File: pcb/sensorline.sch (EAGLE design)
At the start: 31 parts, among them X1 52745-1290

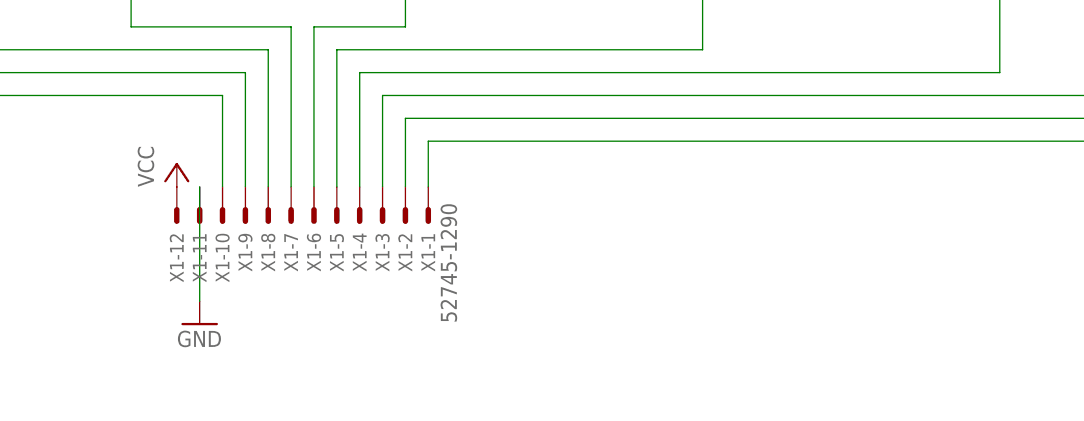
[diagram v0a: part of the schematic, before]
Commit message: a takie tam poprawki
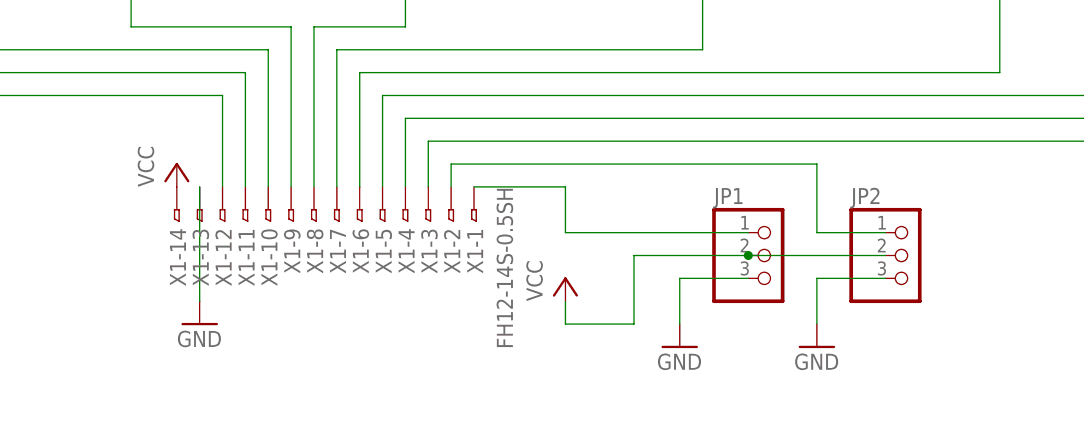
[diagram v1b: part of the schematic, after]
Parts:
- added JP1, JP2: (no value), pinhead:PINHD-1X3
- X1: value 52745-1290 -> FH12-14S-0.5SH; device con-molex:52745-1290 -> con-hirose:FH12-14S-0.5SH
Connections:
- new net N$21: JP1.1, X1-1.1
- new net N$22: JP2.1, X1-2.1
- net GND: now also JP1.3, JP2.3, X1-13.1; no longer X1-11.S
- net N$10: now also X1-8.1; no longer X1-6.S
- net N$12: now also X1-7.1; no longer X1-5.S
- net N$14: now also X1-6.1; no longer X1-4.S
- net N$16: now also X1-5.1; no longer X1-3.S
- net N$18: now also X1-4.1; no longer X1-2.S
- net N$2: now also X1-12.1; no longer X1-10.S
- net N$20: now also X1-3.1; no longer X1-1.S
- net N$4: now also X1-11.1; no longer X1-9.S
- net N$6: now also X1-10.1; no longer X1-8.S
- net N$8: now also X1-9.1; no longer X1-7.S
- net VCC: now also JP1.2, JP2.2, X1-14.1; no longer X1-12.S
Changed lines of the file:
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@@
 <?xml version="1.0" encoding="utf-8"?>
 <!DOCTYPE eagle SYSTEM "eagle.dtd">
-<eagle version="7.1.0">
+<eagle version="8.1.1">
 <drawing>
 <settings>
@@
 <part name="GND10" library="supply1" deviceset="GND" device=""/>
 <part name="P+10" library="supply1" deviceset="VCC" device=""/>
-<part name="X1" library="con-molex" deviceset="52745-1290" device=""/>
 <part name="P+11" library="supply1" deviceset="VCC" device=""/>
 <part name="GND11" library="supply1" deviceset="GND" device=""/>
 <part name="FRAME1" library="frames" deviceset="DINA3_L" device=""/>
+<part name="X1" library="con-hirose" deviceset="FH12-14S-0.5S" device="H"/>
+<part name="JP1" library="pinhead" deviceset="PINHD-1X3" device=""/>
+<part name="JP2" library="pinhead" deviceset="PINHD-1X3" device=""/>
+<part name="P+12" library="supply1" deviceset="VCC" device=""/>
+<part name="GND12" library="supply1" deviceset="GND" device=""/>
+<part name="GND13" library="supply1" deviceset="GND" device=""/>
 </parts>
 <sheets>
@@
 <instance part="GND10" gate="1" x="251.46" y="78.74"/>
 <instance part="P+10" gate="VCC" x="251.46" y="119.38"/>
-<instance part="X1" gate="-1" x="109.22" y="45.72" rot="R270"/>
-<instance part="X1" gate="-2" x="106.68" y="45.72" rot="R270"/>
-<instance part="X1" gate="-3" x="104.14" y="45.72" rot="R270"/>
-<instance part="X1" gate="-4" x="101.6" y="45.72" rot="R270"/>
-<instance part="X1" gate="-5" x="99.06" y="45.72" rot="R270"/>
-<instance part="X1" gate="-6" x="96.52" y="45.72" rot="R270"/>
-<instance part="X1" gate="-7" x="93.98" y="45.72" rot="R270"/>
-<instance part="X1" gate="-8" x="91.44" y="45.72" rot="R270"/>
-<instance part="X1" gate="-9" x="88.9" y="45.72" rot="R270"/>
-<instance part="X1" gate="-10" x="86.36" y="45.72" rot="R270"/>
-<instance part="X1" gate="-11" x="83.82" y="45.72" rot="R270"/>
-<instance part="X1" gate="-12" x="81.28" y="45.72" rot="R270"/>
 <instance part="P+11" gate="VCC" x="81.28" y="50.8"/>
 <instance part="GND11" gate="1" x="83.82" y="33.02"/>
 <instance part="FRAME1" gate="G$1" x="-78.74" y="-60.96"/>
 <instance part="FRAME1" gate="G$2" x="208.28" y="-60.96"/>
+<instance part="X1" gate="-1" x="114.3" y="45.72" rot="R270"/>
+<instance part="X1" gate="-2" x="111.76" y="45.72" rot="R270"/>
+<instance part="X1" gate="-3" x="109.22" y="45.72" rot="R270"/>
+<instance part="X1" gate="-4" x="106.68" y="45.72" rot="R270"/>
+<instance part="X1" gate="-5" x="104.14" y="45.72" rot="R270"/>
+<instance part="X1" gate="-6" x="101.6" y="45.72" rot="R270"/>
+<instance part="X1" gate="-7" x="99.06" y="45.72" rot="R270"/>
+<instance part="X1" gate="-8" x="96.52" y="45.72" rot="R270"/>
+<instance part="X1" gate="-9" x="93.98" y="45.72" rot="R270"/>
+<instance part="X1" gate="-10" x="91.44" y="45.72" rot="R270"/>
+<instance part="X1" gate="-11" x="88.9" y="45.72" rot="R270"/>
+<instance part="X1" gate="-12" x="86.36" y="45.72" rot="R270"/>
+<instance part="X1" gate="-13" x="83.82" y="45.72" rot="R270"/>
+<instance part="X1" gate="-14" x="81.28" y="45.72" rot="R270"/>
+<instance part="JP1" gate="A" x="147.32" y="40.64"/>
+<instance part="JP2" gate="A" x="162.56" y="40.64"/>
+<instance part="P+12" gate="VCC" x="124.46" y="38.1"/>
+<instance part="GND12" gate="1" x="137.16" y="30.48"/>
+<instance part="GND13" gate="1" x="152.4" y="30.48"/>
 </instances>
 <busses>
@@
 <junction x="-38.1" y="99.06"/>
 <wire x1="-25.4" y1="99.06" x2="-25.4" y2="58.42" width="0.1524" layer="91"/>
-<pinref part="X1" gate="-10" pin="S"/>
 <wire x1="-25.4" y1="58.42" x2="86.36" y2="58.42" width="0.1524" layer="91"/>
 <wire x1="86.36" y1="58.42" x2="86.36" y2="48.26" width="0.1524" layer="91"/>
+<pinref part="X1" gate="-12" pin="1"/>
 </segment>
 </net>
@@
 </segment>
 <segment>
-<pinref part="X1" gate="-11" pin="S"/>
 <pinref part="GND11" gate="1" pin="GND"/>
 <wire x1="83.82" y1="48.26" x2="83.82" y2="35.56" width="0.1524" layer="91"/>
+<pinref part="X1" gate="-13" pin="1"/>
+</segment>
+<segment>
+<pinref part="JP1" gate="A" pin="3"/>
+<wire x1="144.78" y1="38.1" x2="137.16" y2="38.1" width="0.1524" layer="91"/>
+<wire x1="137.16" y1="38.1" x2="137.16" y2="33.02" width="0.1524" layer="91"/>
+<pinref part="GND12" gate="1" pin="GND"/>
+</segment>
+<segment>
+<pinref part="JP2" gate="A" pin="3"/>
+<wire x1="160.02" y1="38.1" x2="152.4" y2="38.1" width="0.1524" layer="91"/>
+<wire x1="152.4" y1="38.1" x2="152.4" y2="33.02" width="0.1524" layer="91"/>
+<pinref part="GND13" gate="1" pin="GND"/>
 </segment>
 </net>
@@
 </segment>
 <segment>
-<pinref part="X1" gate="-12" pin="S"/>
 <pinref part="P+11" gate="VCC" pin="VCC"/>
+<pinref part="X1" gate="-14" pin="1"/>
+</segment>
+<segment>
+<pinref part="JP2" gate="A" pin="2"/>
+<pinref part="JP1" gate="A" pin="2"/>
+<wire x1="160.02" y1="40.64" x2="144.78" y2="40.64" width="0.1524" layer="91"/>
+<wire x1="144.78" y1="40.64" x2="132.08" y2="40.64" width="0.1524" layer="91"/>
+<wire x1="132.08" y1="40.64" x2="132.08" y2="33.02" width="0.1524" layer="91"/>
+<junction x="144.78" y="40.64"/>
+<wire x1="132.08" y1="33.02" x2="124.46" y2="33.02" width="0.1524" layer="91"/>
+<wire x1="124.46" y1="33.02" x2="124.46" y2="35.56" width="0.1524" layer="91"/>
+<pinref part="P+12" gate="VCC" pin="VCC"/>
 </segment>
 </net>
@@
 <junction x="-5.08" y="99.06"/>
 <wire x1="7.62" y1="99.06" x2="7.62" y2="60.96" width="0.1524" layer="91"/>
-<pinref part="X1" gate="-9" pin="S"/>
 <wire x1="7.62" y1="60.96" x2="88.9" y2="60.96" width="0.1524" layer="91"/>
 <wire x1="88.9" y1="60.96" x2="88.9" y2="48.26" width="0.1524" layer="91"/>
+<pinref part="X1" gate="-11" pin="1"/>
 </segment>
 </net>
@@
 <junction x="27.94" y="99.06"/>
 <wire x1="40.64" y1="99.06" x2="40.64" y2="63.5" width="0.1524" layer="91"/>
-<pinref part="X1" gate="-8" pin="S"/>
 <wire x1="40.64" y1="63.5" x2="91.44" y2="63.5" width="0.1524" layer="91"/>
 <wire x1="91.44" y1="63.5" x2="91.44" y2="48.26" width="0.1524" layer="91"/>
+<pinref part="X1" gate="-10" pin="1"/>
 </segment>
 </net>
@@
 <junction x="60.96" y="99.06"/>
 <wire x1="76.2" y1="99.06" x2="76.2" y2="66.04" width="0.1524" layer="91"/>
-<pinref part="X1" gate="-7" pin="S"/>
 <wire x1="76.2" y1="66.04" x2="93.98" y2="66.04" width="0.1524" layer="91"/>
 <wire x1="93.98" y1="66.04" x2="93.98" y2="48.26" width="0.1524" layer="91"/>
+<pinref part="X1" gate="-9" pin="1"/>
 </segment>
 </net>
@@
 <junction x="93.98" y="99.06"/>
 <wire x1="106.68" y1="99.06" x2="106.68" y2="66.04" width="0.1524" layer="91"/>
-<pinref part="X1" gate="-6" pin="S"/>
 <wire x1="106.68" y1="66.04" x2="96.52" y2="66.04" width="0.1524" layer="91"/>
 <wire x1="96.52" y1="66.04" x2="96.52" y2="48.26" width="0.1524" layer="91"/>
+<pinref part="X1" gate="-8" pin="1"/>
 </segment>
 </net>
@@
 <junction x="127" y="99.06"/>
 <wire x1="139.7" y1="99.06" x2="139.7" y2="63.5" width="0.1524" layer="91"/>
-<pinref part="X1" gate="-5" pin="S"/>
 <wire x1="139.7" y1="63.5" x2="99.06" y2="63.5" width="0.1524" layer="91"/>
 <wire x1="99.06" y1="63.5" x2="99.06" y2="48.26" width="0.1524" layer="91"/>
+<pinref part="X1" gate="-7" pin="1"/>
 </segment>
 </net>
@@
 <wire x1="172.72" y1="60.96" x2="101.6" y2="60.96" width="0.1524" layer="91"/>
 <wire x1="101.6" y1="60.96" x2="101.6" y2="48.26" width="0.1524" layer="91"/>
-<pinref part="X1" gate="-4" pin="S"/>
+<pinref part="X1" gate="-6" pin="1"/>
 </segment>
 </net>
@@
 <junction x="193.04" y="99.06"/>
 <wire x1="205.74" y1="99.06" x2="205.74" y2="58.42" width="0.1524" layer="91"/>
-<pinref part="X1" gate="-3" pin="S"/>
 <wire x1="205.74" y1="58.42" x2="104.14" y2="58.42" width="0.1524" layer="91"/>
 <wire x1="104.14" y1="58.42" x2="104.14" y2="48.26" width="0.1524" layer="91"/>
+<pinref part="X1" gate="-5" pin="1"/>
 </segment>
 </net>
@@
 <junction x="226.06" y="99.06"/>
 <wire x1="238.76" y1="99.06" x2="238.76" y2="55.88" width="0.1524" layer="91"/>
-<pinref part="X1" gate="-2" pin="S"/>
 <wire x1="238.76" y1="55.88" x2="106.68" y2="55.88" width="0.1524" layer="91"/>
 <wire x1="106.68" y1="55.88" x2="106.68" y2="48.26" width="0.1524" layer="91"/>
+<pinref part="X1" gate="-4" pin="1"/>
 </segment>
 </net>
@@
 <junction x="259.08" y="99.06"/>
 <wire x1="271.78" y1="99.06" x2="271.78" y2="53.34" width="0.1524" layer="91"/>
-<pinref part="X1" gate="-1" pin="S"/>
 <wire x1="271.78" y1="53.34" x2="109.22" y2="53.34" width="0.1524" layer="91"/>
 <wire x1="109.22" y1="53.34" x2="109.22" y2="48.26" width="0.1524" layer="91"/>
-</segment>
-</net>
+<pinref part="X1" gate="-3" pin="1"/>
+</segment>
+</net>
+<net name="N$21" class="0">
+<segment>
+<pinref part="JP1" gate="A" pin="1"/>
+<wire x1="144.78" y1="43.18" x2="124.46" y2="43.18" width="0.1524" layer="91"/>
+<wire x1="124.46" y1="43.18" x2="124.46" y2="48.26" width="0.1524" layer="91"/>
+<pinref part="X1" gate="-1" pin="1"/>
+<wire x1="124.46" y1="48.26" x2="114.3" y2="48.26" width="0.1524" layer="91"/>
+</segment>
+</net>
+<net name="N$22" class="0">
+<segment>
+<pinref part="JP2" gate="A" pin="1"/>
+<wire x1="160.02" y1="43.18" x2="152.4" y2="43.18" width="0.1524" layer="91"/>
+<wire x1="152.4" y1="43.18" x2="152.4" y2="50.8" width="0.1524" layer="91"/>
+<wire x1="152.4" y1="50.8" x2="111.76" y2="50.8" width="0.1524" layer="91"/>
+<pinref part="X1" gate="-2" pin="1"/>
+<wire x1="111.76" y1="50.8" x2="111.76" y2="48.26" width="0.1524" layer="91"/>
+</segment>
+</net>

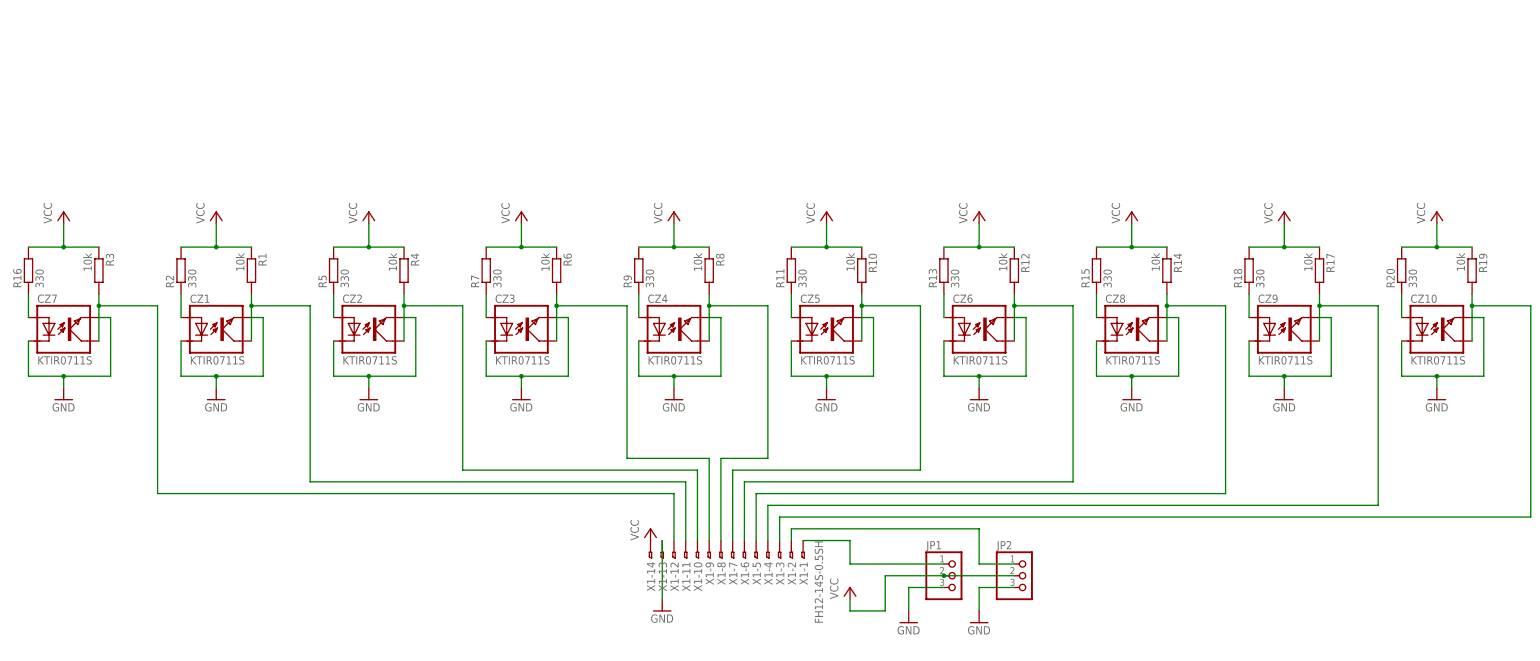
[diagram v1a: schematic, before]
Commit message: o już niewiele
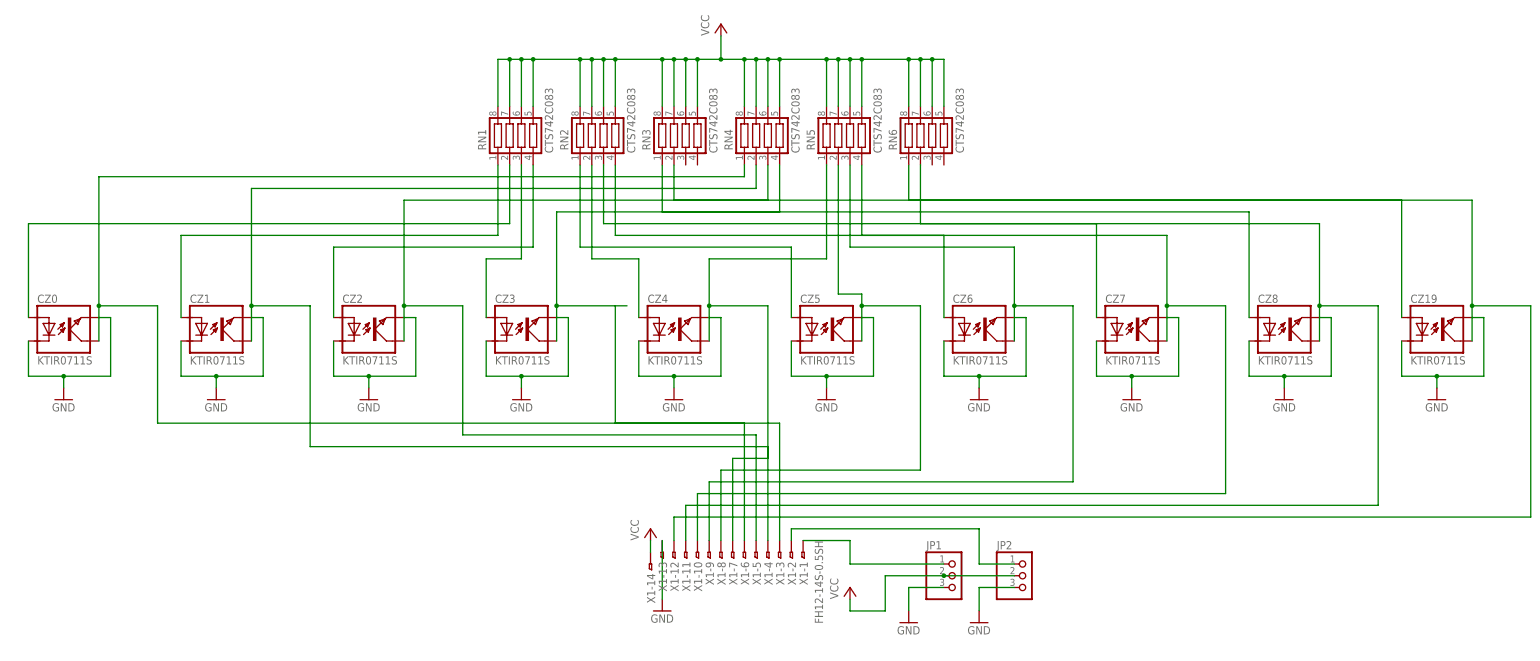
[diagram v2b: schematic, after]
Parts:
- removed CZ9: KTIR0711S, KTIR0711S:KTIR0711S
- removed R1, R10, R12, R14, R17, R19, R3, R4, R6, R8: 10k, rcl:R-EU_R0402
- removed R11, R13, R15, R16, R18, R2, R20, R5, R7, R9: 330, rcl:R-EU_R0402
- added CZ0: KTIR0711S, KTIR0711S:KTIR0711S
- added RN1, RN2, RN3, RN4, RN5, RN6: CTS742C083, resistor-net:CTS742C083
- renumbered CZ10 to CZ19
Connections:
- net GND: now also CZ0.EMITER, CZ0.KATODA; no longer CZ9.EMITER, CZ9.KATODA
- net N$1: now also CZ0.ANODA, RN1.2; no longer CZ7.ANODA, R16.1
- net N$10: now also RN5.1, X1-7.1; no longer R8.2, X1-8.1
- net N$11: now also RN2.1; no longer R11.1
- net N$12: now also RN5.2, X1-8.1; no longer R10.2, X1-7.1
- net N$13: now also RN2.4; no longer R13.1
- net N$14: now also RN5.3, X1-9.1; no longer R12.2, X1-6.1
- net N$15: now also CZ7.ANODA, RN2.3; no longer CZ8.ANODA, R15.1
- net N$16: now also CZ7.KOLEKTOR, RN5.4, X1-10.1; no longer CZ8.KOLEKTOR, R14.2, X1-5.1
- net N$17: now also CZ8.ANODA, RN3.1; no longer CZ9.ANODA, R18.1
- net N$18: now also CZ8.KOLEKTOR, RN6.2, X1-11.1; no longer CZ9.KOLEKTOR, R17.2, X1-4.1
- net N$19: now also RN3.2; no longer R20.1
- net N$2: now also CZ0.KOLEKTOR, RN4.1, X1-3.1; no longer CZ7.KOLEKTOR, R3.2, X1-12.1
- net N$20: now also RN6.1, X1-12.1; no longer R19.2, X1-3.1
- net N$3: now also RN1.1; no longer R2.1
- net N$4: now also RN4.2, X1-4.1; no longer R1.2, X1-11.1
- net N$5: now also RN1.4; no longer R5.1
- net N$6: now also RN4.3, X1-5.1; no longer R4.2, X1-10.1
- net N$7: now also RN1.3; no longer R7.1
- net N$8: now also RN4.4, X1-6.1; no longer R6.2, X1-9.1
- net N$9: now also RN2.2; no longer R9.1
- net VCC: now also RN1.5, RN1.6, RN1.7, RN1.8, RN2.5, RN2.6, RN2.7, RN2.8, RN3.5, RN3.6, RN3.7, RN3.8, RN4.5, RN4.6, RN4.7, RN4.8, RN5.5, RN5.6, RN5.7, RN5.8, RN6.5, RN6.6, RN6.7, RN6.8; no longer R1.1, R10.1, R11.2, R12.1, R13.2, R14.1, R15.2, R16.2, R17.1, R18.2, R19.1, R2.2, R20.2, R3.1, R4.1, R5.2, R6.1, R7.2, R8.1, R9.2
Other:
- moved on the sheet: CZ7, CZ8, X1-14
